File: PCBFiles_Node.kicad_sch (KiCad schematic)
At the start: 33 parts, among them J1 Input, J2 SWD, J3 SPEC Sensor 968-001, J4 SHT31, J5 USB-TTL, J7 SMA, SW1 SW_Push, U1 STM32L431RCTx, U2 RFM9X, U3 STLQ015M33R, Y1 Q13FC1350000400 32.768kHz

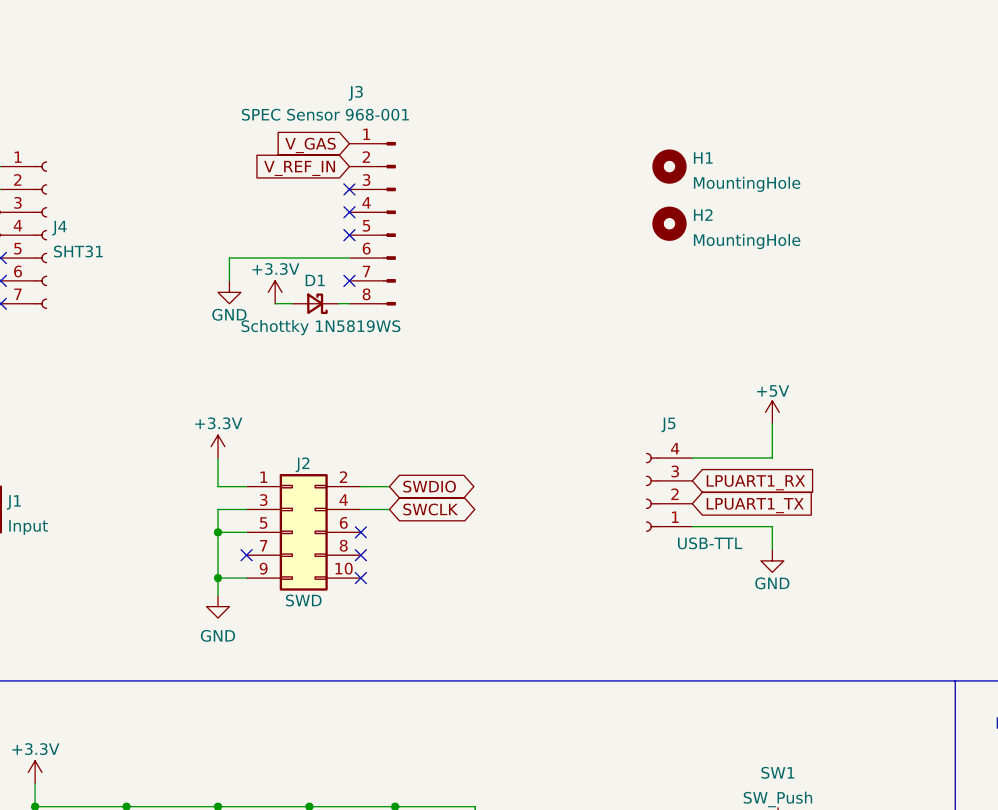
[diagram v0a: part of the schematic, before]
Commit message: First routing
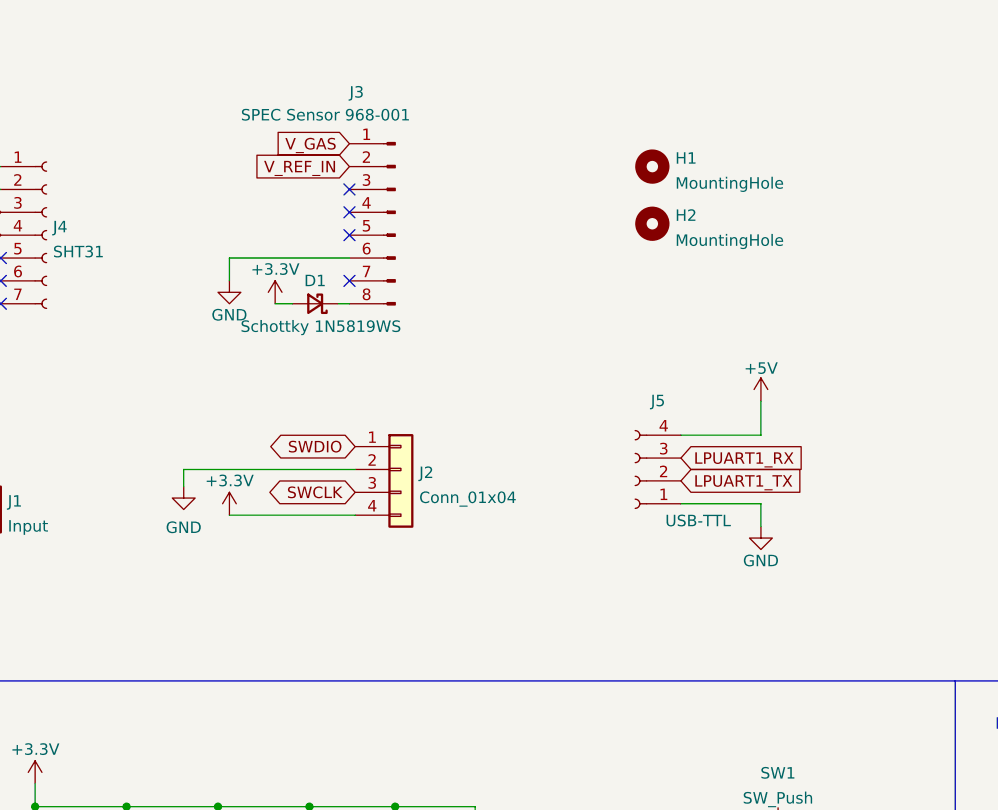
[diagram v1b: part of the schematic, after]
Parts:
- removed J2: SWD, Connector_PinHeader_2.54mm:PinHeader_2x05_P2.54mm_Vertical_SMD, symbol Connector_Generic:Conn_02x05_Odd_Even
- added J2: Conn_01x04, Connector_PinSocket_2.54mm:PinSocket_1x04_P2.54mm_Vertical, symbol Connector_Generic:Conn_01x04
- D2, D3: footprint LED_SMD:LED_0201_0603Metric -> LED_SMD:LED_0603_1608Metric
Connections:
- net +3V3: now also J2.4 (Pin_4)
- net GND: now also J2.2 (Pin_2)
- net SWCLK: now also J2.3 (Pin_3)
- net SWDIO: now also J2.1 (Pin_1)
- no-connect marks 49 -> 45
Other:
- moved on the sheet: H1, H2, J5
